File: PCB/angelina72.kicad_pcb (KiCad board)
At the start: 2 copper layers, 176.4 x 111.6 mm, 88 parts, among them J1 MJ-4PP-9, J2 LED, SW1 KEY_SWITCH, SW10 KEY_SWITCH, SW11 KEY_SWITCH, SW12 KEY_SWITCH, SW13 KEY_SWITCH, SW14 KEY_SWITCH, SW15 KEY_SWITCH, SW16 KEY_SWITCH, SW17 KEY_SWITCH, SW18 KEY_SWITCH, SW19 KEY_SWITCH, SW2 KEY_SWITCH, SW20 KEY_SWITCH, SW21 KEY_SWITCH, SW22 KEY_SWITCH, SW23 KEY_SWITCH, SW24 KEY_SWITCH, SW25 KEY_SWITCH, SW26 KEY_SWITCH, SW27 KEY_SWITCH, SW28 KEY_SWITCH, SW29 KEY_SWITCH, SW3 KEY_SWITCH, SW30 KEY_SWITCH, SW31 KEY_SWITCH, SW32 KEY_SWITCH, SW33 KEY_SWITCH, SW34 KEY_SWITCH, SW35 KEY_SWITCH, SW36 KEY_SWITCH, SW4 KEY_SWITCH, SW5 KEY_SWITCH, SW6 KEY_SWITCH, SW7 KEY_SWITCH, SW8 KEY_SWITCH, SW9 KEY_SWITCH, U1 ProMicro

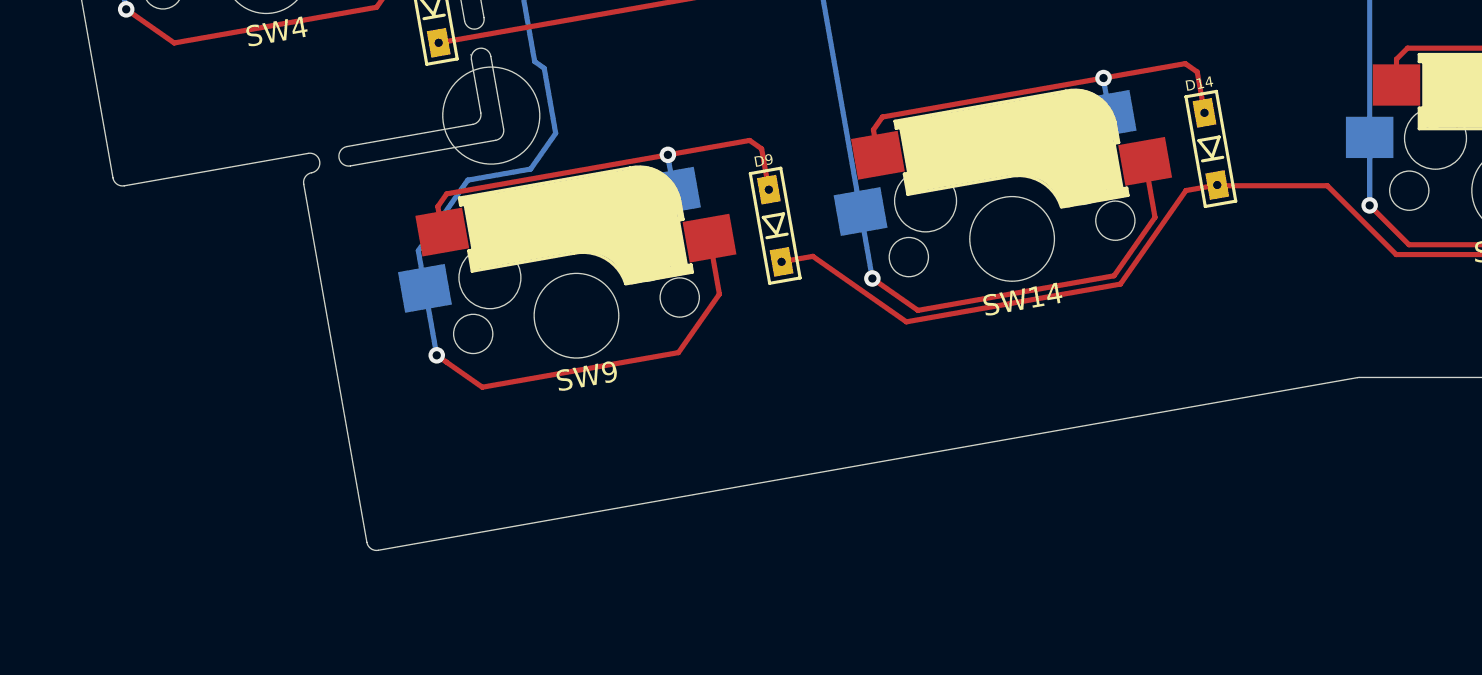
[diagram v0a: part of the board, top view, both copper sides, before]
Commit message: Update PCB, top plate
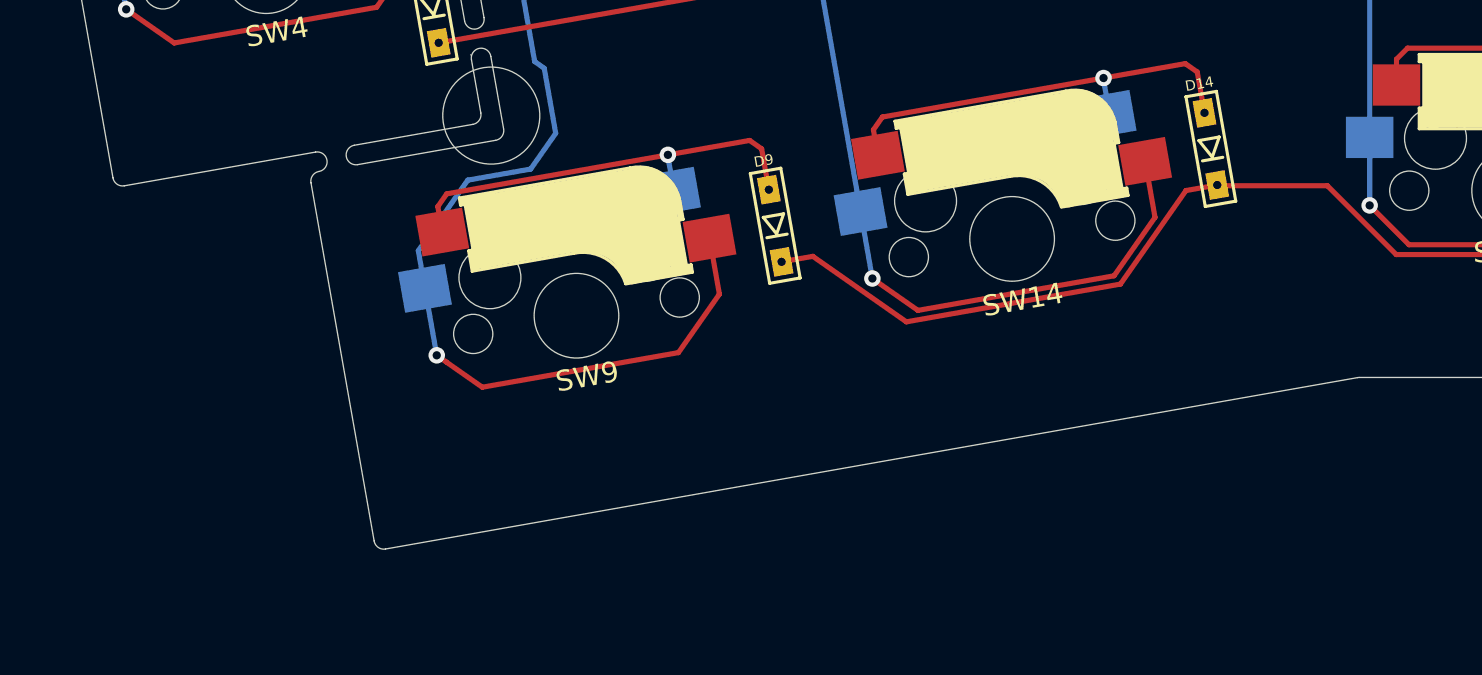
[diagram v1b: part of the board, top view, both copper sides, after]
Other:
- outline, holes or cut-outs redrawn
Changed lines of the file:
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@@
   (gr_arc (start 65.649991 79.032478) (end 66.119003 78.949782) (angle -180) (layer Edge.Cuts) (width 0.05))
   (gr_arc (start 65.319197 77.156422) (end 64.850181 77.239123) (angle -180) (layer Edge.Cuts) (width 0.05))
-  (gr_line (start 74.6796 119.271451) (end 68.582435 120.346568) (layer Edge.Cuts) (width 0.05))
-  (gr_arc (start 68.665108 120.815566) (end 68.582435 120.346568) (angle -180.0026468) (layer Edge.Cuts) (width 0.05))
-  (gr_arc (start 66.789075 121.146382) (end 66.87175 121.615378) (angle -180.0026468) (layer Edge.Cuts) (width 0.05))
+  (gr_line (start 74.6796 119.271451) (end 68.934197 120.284543) (layer Edge.Cuts) (width 0.05))
+  (gr_arc (start 69.016871 120.753541) (end 68.934197 120.284543) (angle -180.0026468) (layer Edge.Cuts) (width 0.05))
+  (gr_arc (start 67.140837 121.084357) (end 67.223513 121.553353) (angle -180.0026468) (layer Edge.Cuts) (width 0.05))
   (gr_arc (start 188.469026 37.71159) (end 188.945278 37.71159) (angle -90) (layer Edge.Cuts) (width 0.05))
   (gr_arc (start 189.421526 45.80784) (end 188.945276 45.80784) (angle -90.00336866) (layer Edge.Cuts) (width 0.05))
@@
   (gr_line (start 188.945278 37.71159) (end 188.945276 45.80784) (layer Edge.Cuts) (width 0.05))
   (gr_line (start 110.18339 37.235327) (end 188.469026 37.23534) (layer Edge.Cuts) (width 0.05))
-  (gr_arc (start 70.014347 139.437938) (end 69.545332 139.52064) (angle -90) (layer Edge.Cuts) (width 0.05))
+  (gr_arc (start 70.36611 139.375912) (end 69.897094 139.458614) (angle -90) (layer Edge.Cuts) (width 0.05))
   (gr_arc (start 91.685142 39.501907) (end 91.623117 39.150143) (angle -90.00016041) (layer Edge.Cuts) (width 0.05))
   (gr_arc (start 90.981305 39.626012) (end 91.043696 39.978029) (angle -89.94903567) (layer Edge.Cuts) (width 0.05))
@@
   (gr_arc (start 39.111605 67.027821) (end 38.64259 67.110521) (angle -90) (layer Edge.Cuts) (width 0.05))
   (gr_arc (start 36.134407 50.143292) (end 36.051709 49.674278) (angle -90) (layer Edge.Cuts) (width 0.05))
-  (gr_arc (start 66.954449 122.084395) (end 66.871749 121.615379) (angle -90) (layer Edge.Cuts) (width 0.05))
+  (gr_arc (start 67.306212 122.02237) (end 67.223512 121.553354) (angle -90) (layer Edge.Cuts) (width 0.05))
   (gr_arc (start 57.71237 121.779635) (end 57.243356 121.862334) (angle -90) (layer Edge.Cuts) (width 0.05))
-  (gr_line (start 66.706377 120.677387) (end 57.795072 122.248649) (layer Edge.Cuts) (width 0.05))
+  (gr_line (start 67.05814 120.615365) (end 57.795072 122.248649) (layer Edge.Cuts) (width 0.05))
   (gr_arc (start 74.596899 118.802437) (end 74.6796 119.271451) (angle -90) (layer Edge.Cuts) (width 0.05))
   (gr_arc (start 75.700329 119.575067) (end 75.783028 120.044081) (angle -90) (layer Edge.Cuts) (width 0.05))
@@
   (gr_arc (start 62.189618 64.892932) (end 62.658632 64.810231) (angle -90) (layer Edge.Cuts) (width 0.05))
   (gr_arc (start 62.96225 63.789501) (end 63.431262 63.706802) (angle -90) (layer Edge.Cuts) (width 0.05))
-  (gr_line (start 75.783028 120.044081) (end 68.747804 121.28456) (layer Edge.Cuts) (width 0.05))
+  (gr_line (start 75.783028 120.044081) (end 69.099566 121.222535) (layer Edge.Cuts) (width 0.05))
   (gr_line (start 72.861344 100.731779) (end 75.218296 114.098697) (layer Edge.Cuts) (width 0.05))
   (gr_line (start 67.384976 101.213813) (end 72.309631 100.345462) (layer Edge.Cuts) (width 0.05))
@@
   (gr_line (start 56.61753 59.346881) (end 54.75678 48.794054) (layer Edge.Cuts) (width 0.05))
   (gr_line (start 53.81875 48.959451) (end 55.679498 59.512286) (layer Edge.Cuts) (width 0.05))
-  (gr_line (start 70.097047 139.906952) (end 117.542847 131.540747) (layer Edge.Cuts) (width 0.05))
-  (gr_line (start 66.485435 122.167095) (end 69.545332 139.52064) (layer Edge.Cuts) (width 0.05))
+  (gr_line (start 70.448812 139.844928) (end 117.542847 131.540747) (layer Edge.Cuts) (width 0.05))
+  (gr_line (start 66.837197 122.10507) (end 69.897094 139.458614) (layer Edge.Cuts) (width 0.05))
   (gr_line (start 54.100759 104.039777) (end 57.243356 121.862334) (layer Edge.Cuts) (width 0.05))
   (gr_line (start 48.624392 104.521811) (end 53.549043 103.653463) (layer Edge.Cuts) (width 0.05))
@@
   (segment (start 39.022628 57.467424) (end 37.94025 59.013216) (width 0.25) (layer B.Cu) (net 48))
   (segment (start 38.723626 55.771707) (end 39.022628 57.467424) (width 0.25) (layer B.Cu) (net 48))
-  (via (at 38.312406 61.12381) (size 0.8) (drill 0.4) (layers F.Cu B.Cu) (net 48) (status 1000000))
+  (via (at 38.312406 61.12381) (size 0.8) (drill 0.4) (layers F.Cu B.Cu) (net 48))
   (segment (start 44.463949 65.842279) (end 40.587526 66.525797) (width 0.25) (layer B.Cu) (net 48))
   (segment (start 39.078625 65.469253) (end 38.312406 61.12381) (width 0.25) (layer B.Cu) (net 48))

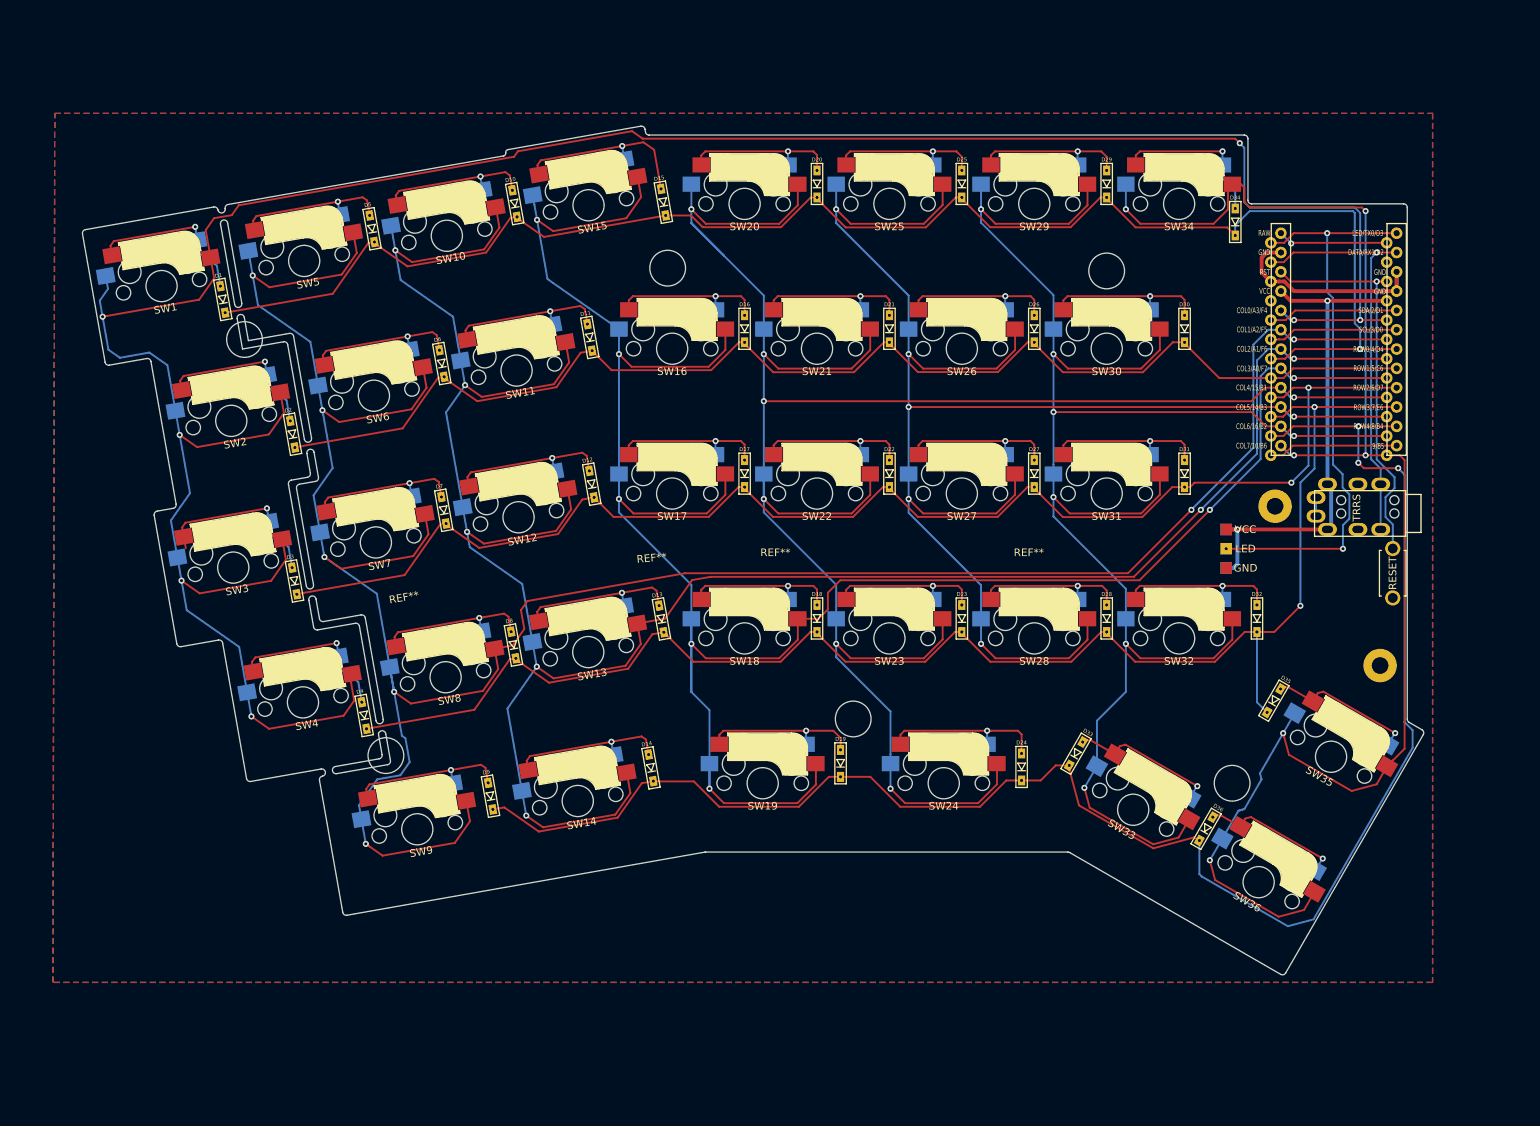
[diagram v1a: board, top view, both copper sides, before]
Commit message: Update PCB, top plate
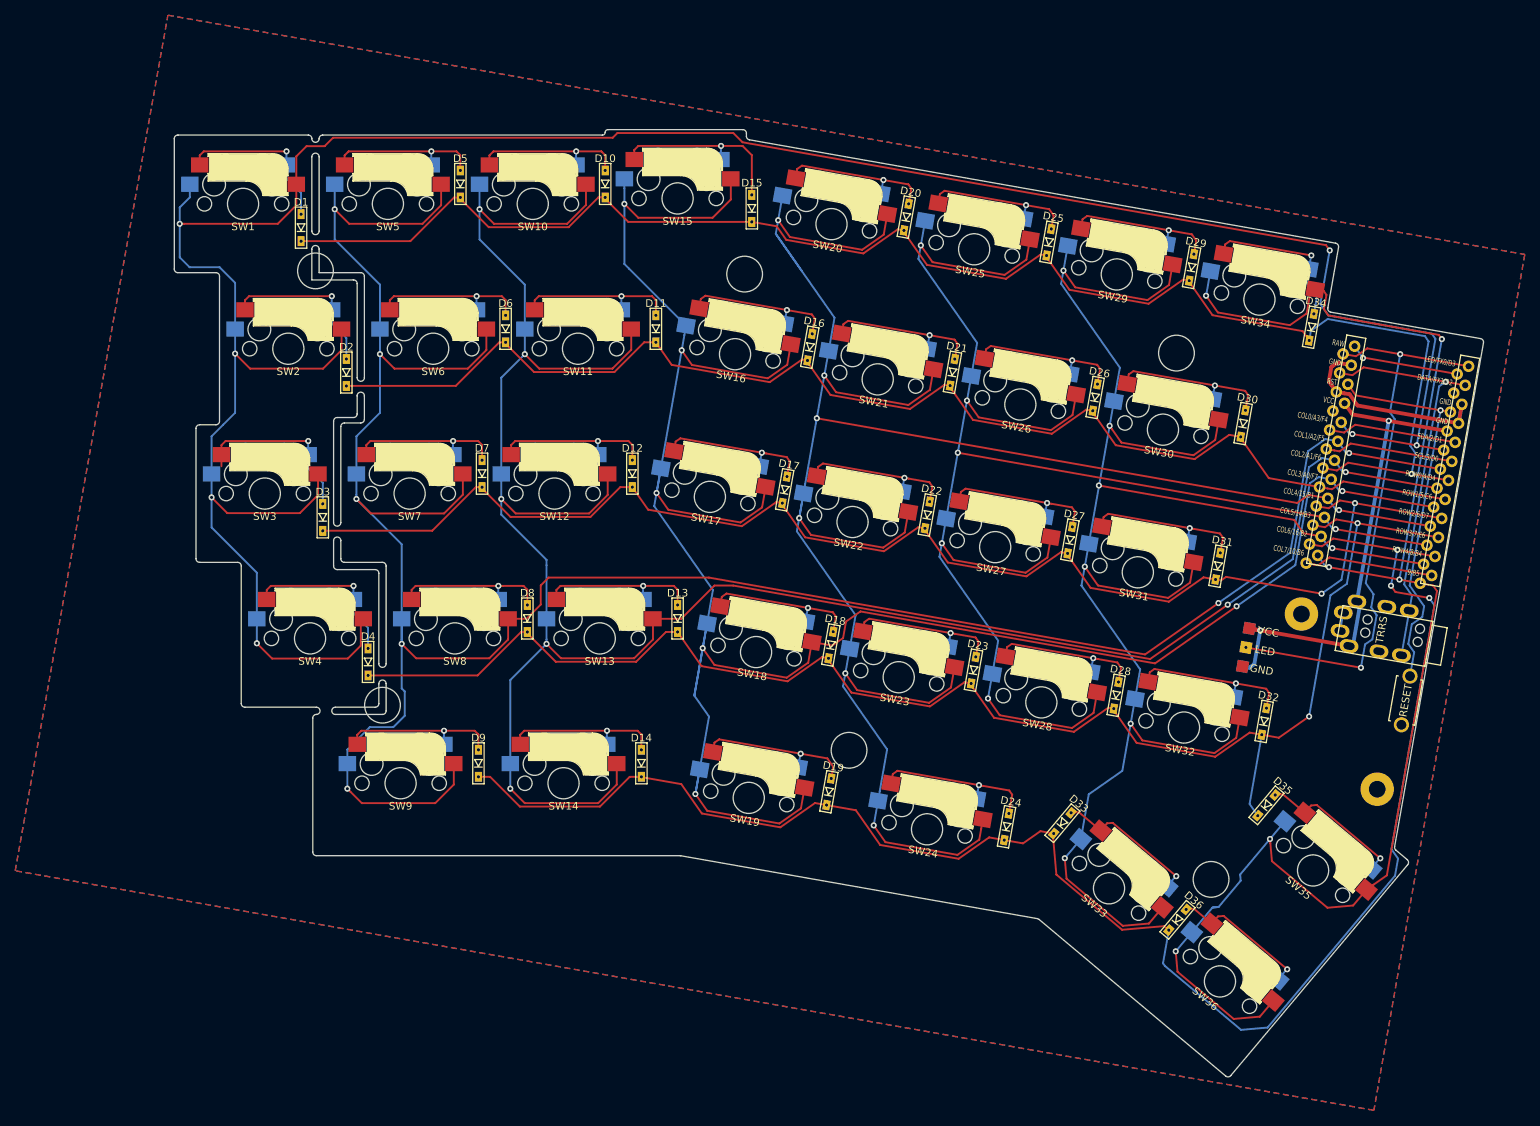
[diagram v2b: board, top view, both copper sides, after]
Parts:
- removed the REF** at (126.8, 91.6)
- removed the REF** at (110.5, 92.4)
- removed the REF** at (77.9, 97.6)
- removed the REF** at (160.1, 91.6)
- moved U1 17.4 mm to (207.9, 80.6), turned to 350 degrees
- moved D34 17.1 mm to (197.3, 62.5), turned to 350 degrees
- moved RSW1 16.8 mm to (209.7, 111.6), turned to 80 degrees
- moved SW34 16.4 mm to (190.5, 58.9), turned to 350 degrees
- moved J1 16.4 mm to (206.8, 103.1), turned to 260 degrees
- moved REF** 16.3 mm to (205.9, 123.3), turned to 350 degrees
- moved D29 15.7 mm to (181.5, 54.6), turned to 350 degrees
- moved SW1 15.2 mm to (56.8, 46.3), turned to 0 degrees
- moved SW35 15.1 mm to (197.5, 134.0), turned to 320 degrees
- moved D30 14.7 mm to (188.3, 75.2), turned to 350 degrees
- moved REF** 14.6 mm to (196.0, 100.2), turned to 350 degrees
- moved SW29 14.3 mm to (171.7, 55.6), turned to 350 degrees
- moved REF** 14.2 mm to (179.5, 65.9), turned to 0 degrees
- moved SW36 14.0 mm to (185.3, 148.5), turned to 320 degrees
- moved D1 14.0 mm to (64.4, 49.4), turned to 0 degrees
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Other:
- board size 176.4 x 111.6 mm -> 172.2 x 124.6 mm
